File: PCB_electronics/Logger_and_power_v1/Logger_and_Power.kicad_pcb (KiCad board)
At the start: 2 copper layers, 97.5 x 90 mm, 41 parts, among them IC1 ATMEGA328-P, P1 SOLAR_PANEL, P10 CONN_01X08, P11 CONN_01X08, P12 CONN_01X03, P13 CONN_01X02, P14 CONN_01X02, P15 CONN_01X02, P2 5V_pololu, P3 BATT, P4 SUPERCAPS, P5 GPS_breakout_connector, P6 SD_breakout_connector, P7 Iridium_connector, P8 VN100_connector, P9 RPI_connector, U1 IRLB_8721_SOL, U2 IRLS-8721_MEGA, U3 MAX232, U4 FQP27P06, Y1 16MHz

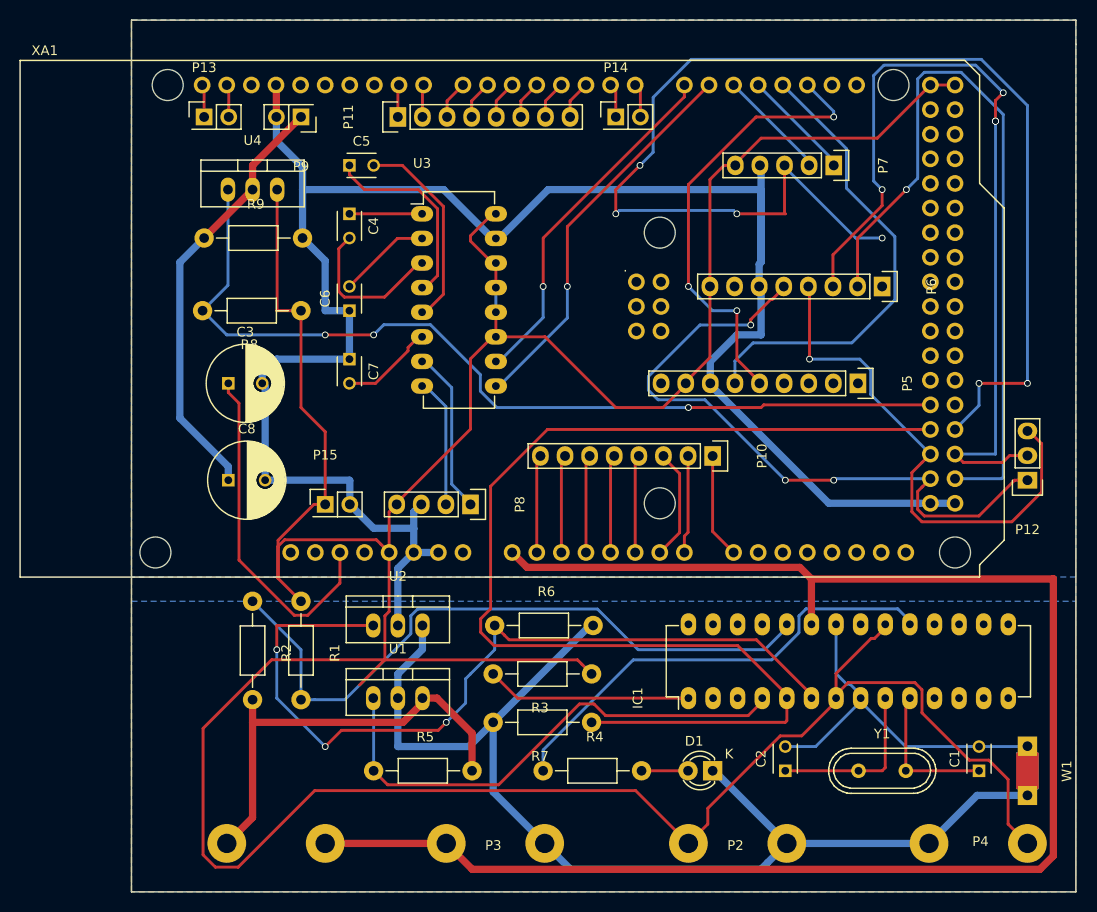
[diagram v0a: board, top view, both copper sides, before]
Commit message: ready to try to shift the power controller
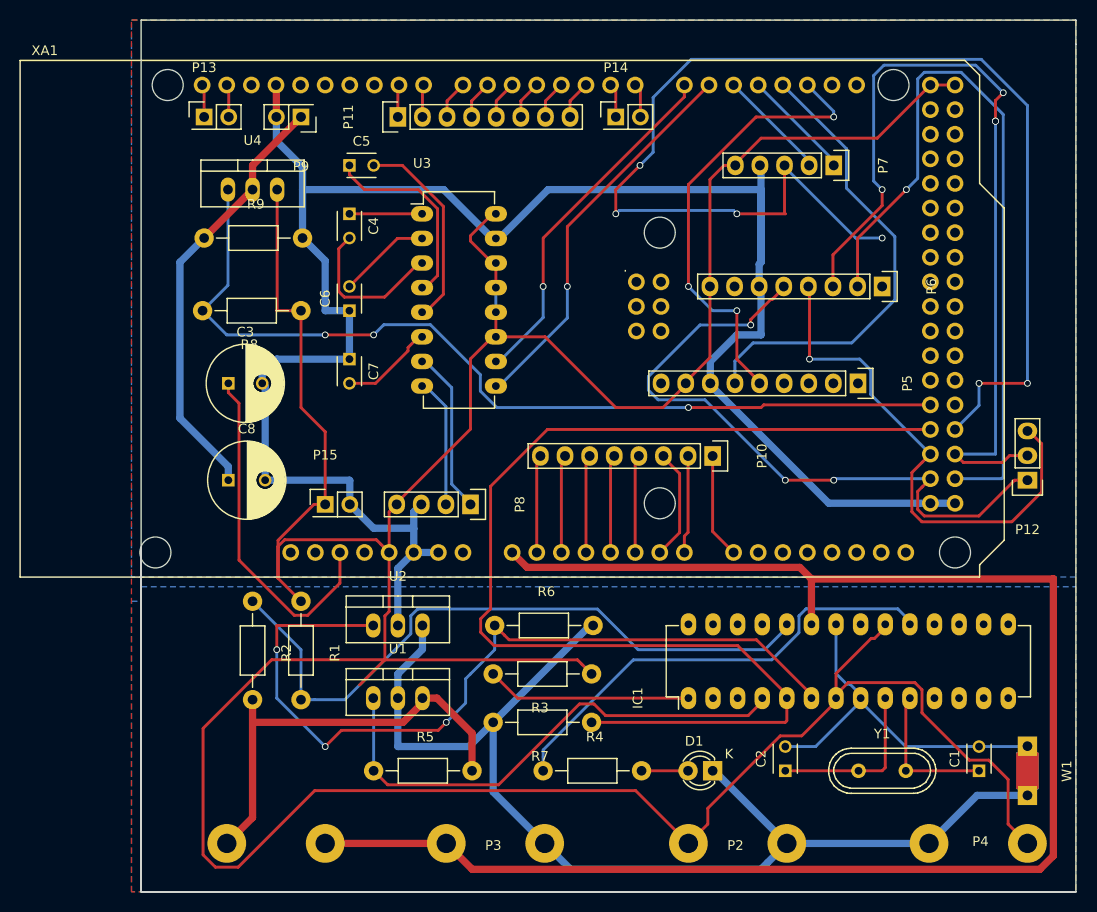
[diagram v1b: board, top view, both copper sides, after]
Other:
- board size 97.5 x 90 mm -> 96.5 x 90 mm
